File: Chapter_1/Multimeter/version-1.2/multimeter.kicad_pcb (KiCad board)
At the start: 2 copper layers, 102.4 x 84 mm, 66 parts, among them J1 Screw_Terminal_01x02, J2 Conn_01x02_Socket, J3 Screw_Terminal_01x02, Q1 IRLZ44N, Q17 BC547, Q18 BC547, Q19 BC547, Q20 BC547, Q22 BC547, Q23 BC547, Q24 BC547, Q25 BC547, Q26 BC547, Q27 BC547, Q28 BC547, Q29 BC547, Q30 BC547, Q31 BC547, Q32 BC547, Q33 IRLZ44N, Q34 IRLZ44N, SW1 SW_DPST_x2, SW2 SW_DPST_x2, SW3 SW_DPST_x2

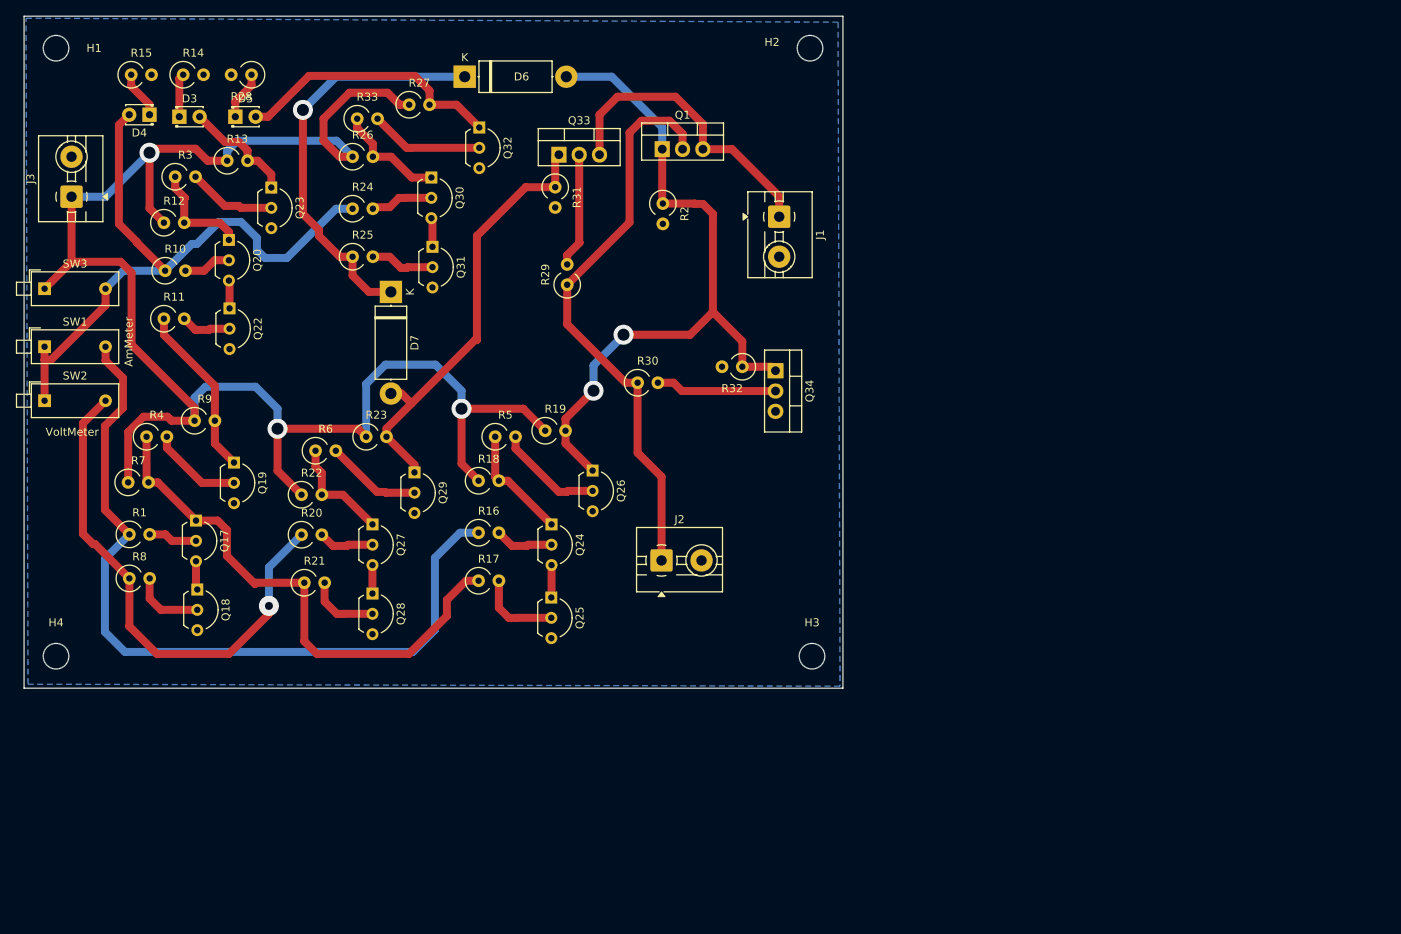
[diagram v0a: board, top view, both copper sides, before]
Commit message: .
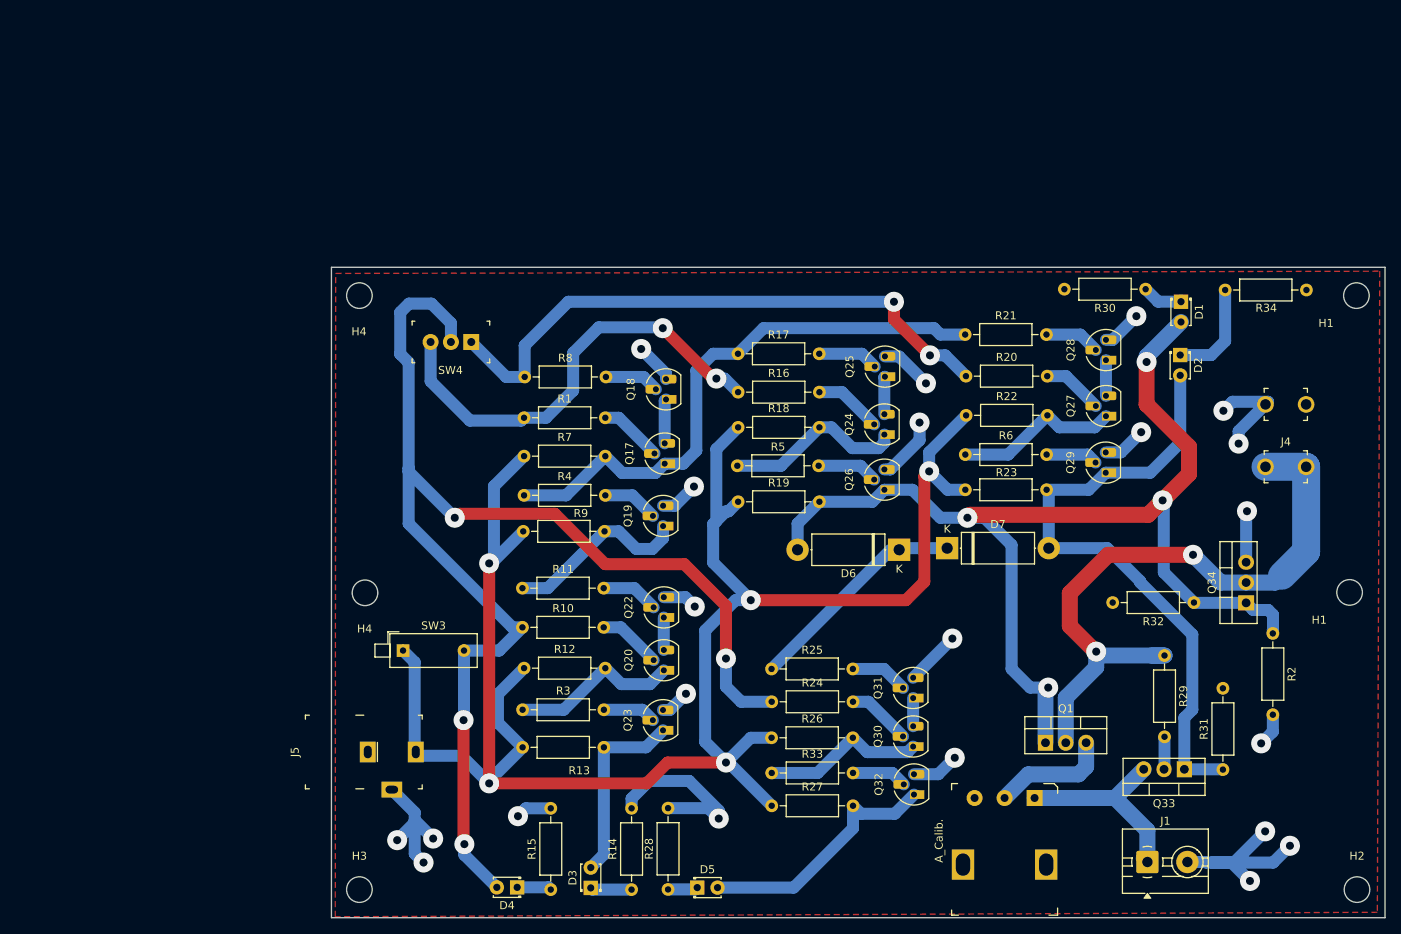
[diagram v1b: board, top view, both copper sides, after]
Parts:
- removed the H1 at (3.81, 3.69)
- removed the H4 at (3.81, 79.7)
- removed J3: Screw_Terminal_01x02, TerminalBlock:TerminalBlock_MaiXu_MX126-5.0-02P_1x02_P5.00mm
- removed SW1, SW2: SW_DPST_x2, Button_Switch_THT:SW_DIP_SPSTx01_Piano_10.8x4.1mm_W7.62mm_P2.54mm
- added A_Calib.: P120PK-Y25BR10K, digikey-footprints:Potentiometer_P120PK-Y25BR10K, F.Cu at (126.1, 97.4)
- added D1: A_METER- LED, LED_THT:LED_D1.8mm_W3.3mm_H2.4mm, F.Cu at (144.4, 35.4)
- added D2: V_METER- LED, LED_THT:LED_D1.8mm_W3.3mm_H2.4mm, F.Cu at (144.3, 42.0)
- added H1: MountingHole, MountingHole:MountingHole_3.2mm_M3, F.Cu at (166.4, 34.6)
- added H1: MountingHole, MountingHole:MountingHole_3.2mm_M3, F.Cu at (165.5, 71.7)
- added H4: MountingHole, MountingHole:MountingHole_3.2mm_M3, F.Cu at (41.7, 34.6)
- added H4: MountingHole, MountingHole:MountingHole_3.2mm_M3, F.Cu at (42.4, 71.8)
- added J4: 105-1102-001, digikey-footprints:Test_Jack_Horiz, F.Cu at (157.5, 56.0)
- added J5: PJ-102A, digikey-footprints:Barrel_Jack_5.5mmODx2.1mmID_PJ-102A, F.Cu at (45.8, 91.7)
- added R34: 1K, Resistor_THT:R_Axial_DIN0207_L6.3mm_D2.5mm_P10.16mm_Horizontal, F.Cu at (150.0, 33.9)
- added SW4: SW_Nidec_CAS-120A1, digikey-footprints:Switch_Toggle_ATE1D-2M3-10-Z, F.Cu at (53.2, 40.4)
- J2: value Conn_01x02_Socket -> 105-1103-001; footprint TerminalBlock:TerminalBlock_MaiXu_MX126-5.0-02P_1x02_P5.00mm -> digikey-footprints:Test_Jack_Horiz
- Q17, Q18, Q19, Q20, Q22, Q23, Q24, Q25, Q26, Q27, Q28, Q29, Q30, Q31, Q32: footprint Package_TO_SOT_THT:TO-92L_Inline_Wide -> Package_TO_SOT_THT:TO-92_HandSolder
- R1, R10, R11, R12, R13, R14, R15, R16, R17, R18, R19, R2, R20, R21, R22, R23, R24, R25, R26, R27, R28, R29, R3, R31, R32, R33, R4, R5, R6, R7, R8, R9: footprint Resistor_THT:R_Axial_DIN0309_L9.0mm_D3.2mm_P2.54mm_Vertical -> Resistor_THT:R_Axial_DIN0207_L6.3mm_D2.5mm_P10.16mm_Horizontal
- R30: value 0.015 Ohm -> 1K; footprint Resistor_THT:R_Axial_DIN0309_L9.0mm_D3.2mm_P2.54mm_Vertical -> Resistor_THT:R_Axial_DIN0207_L6.3mm_D2.5mm_P10.16mm_Horizontal
- moved H2 125.4 mm to (166.4, 108.9)
- moved R14 116.3 mm to (75.8, 108.9), turned to 90 degrees
- moved R15 114.6 mm to (65.7, 108.9), turned to 90 degrees
- moved R28 114.4 mm to (80.3, 108.8), turned to 90 degrees
- moved D5 112.3 mm to (84.0, 108.6)
- moved R31 110.8 mm to (149.7, 93.9), turned to 90 degrees
- moved Q33 109.6 mm to (144.9, 93.8), turned to 180 degrees
- moved D3 109.3 mm to (70.7, 108.7), turned to 90 degrees
- moved D4 107.0 mm to (61.5, 108.6)
- moved Q32 99.5 mm to (111.1, 97.0), turned to 90 degrees
- moved R27 98.7 mm to (93.3, 98.4)
- moved R33 96.8 mm to (93.3, 94.3)
- moved Q28 96.2 mm to (135.1, 42.7), turned to 90 degrees
- moved R2 93.3 mm to (155.9, 76.8)
- moved Q30 93.2 mm to (111.0, 91.0), turned to 90 degrees
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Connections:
- J2 pad 1: /INPUT_POSITIVE -> GND
- Q1 pad 3: Net-(J1-Pin_1) -> Net-(POT1-S)
- Q34 pad 2: Net-(Q34-D) -> /INPUT_POSITIVE
- R30 pad 1: /INPUT_POSITIVE -> Net-(D1-K)
- R30 pad 2: Net-(Q34-D) -> GND
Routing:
- net GND: track 0.00 -> 151.4 mm, vias 0 -> 22
- net /SIGNAL_POWER_BUTTON: track 81.7 -> 160.5 mm, vias 0 -> 4
- net /SIGNAL_MEASURING_AMPS: track 89.8 -> 143.0 mm, vias 2 -> 4
- net /SIGNAL_AMMETER: track 99.2 -> 56.3 mm, vias 0 -> 2
- net VCC: track 211.6 -> 242.5 mm, vias 3 -> 5
- net Net-(D6-K): track 52.5 -> 28.2 mm, vias 1 -> 0
- net /SIGNAL_MEASURING_VOLTS: track 55.5 -> 79.6 mm
- net Net-(Q34-D): track 15.1 -> 0.00 mm
- net Net-(POT1-S): track 0.00 -> 14.8 mm
- net Net-(D2-K): track 0.00 -> 12.7 mm
- net Net-(J1-Pin_1): track 37.9 -> 25.5 mm
- net /SIGNAL_VOLTMETER: track 64.5 -> 75.1 mm, vias 1 -> 2
- net Net-(Q33-D): track 14.4 -> 4.17 mm
- net /INPUT_POSITIVE: track 72.3 -> 82.3 mm, vias 0 -> 2
- net /SIGNAL_NOT_ALLOWED: track 14.8 -> 24.0 mm
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- added copper zone on F.Cu, net GND
- removed copper zone on B.Cu, net GND
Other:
- board size 102.4 x 84 mm -> 131.7 x 81.3 mm
- board text removed: "AmMeter"
- board text removed: "VoltMeter"
